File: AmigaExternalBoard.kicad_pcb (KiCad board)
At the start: 2 copper layers, 132.9 x 40.7 mm, 24 parts, among them J1 Conn_01x24, J2 Conn_01x24, J3 Conn_01x24, SW1 SW_SPDT, SW2 SW_SPDT, SW3 SW_SPDT

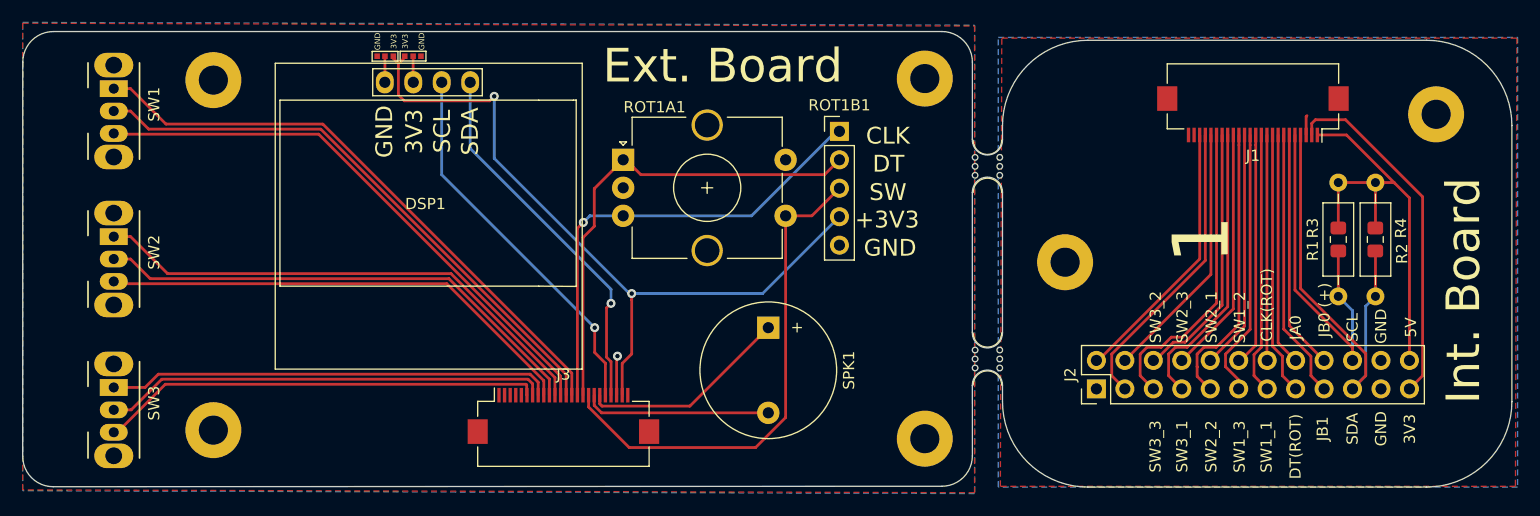
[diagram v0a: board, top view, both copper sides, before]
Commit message: Picture
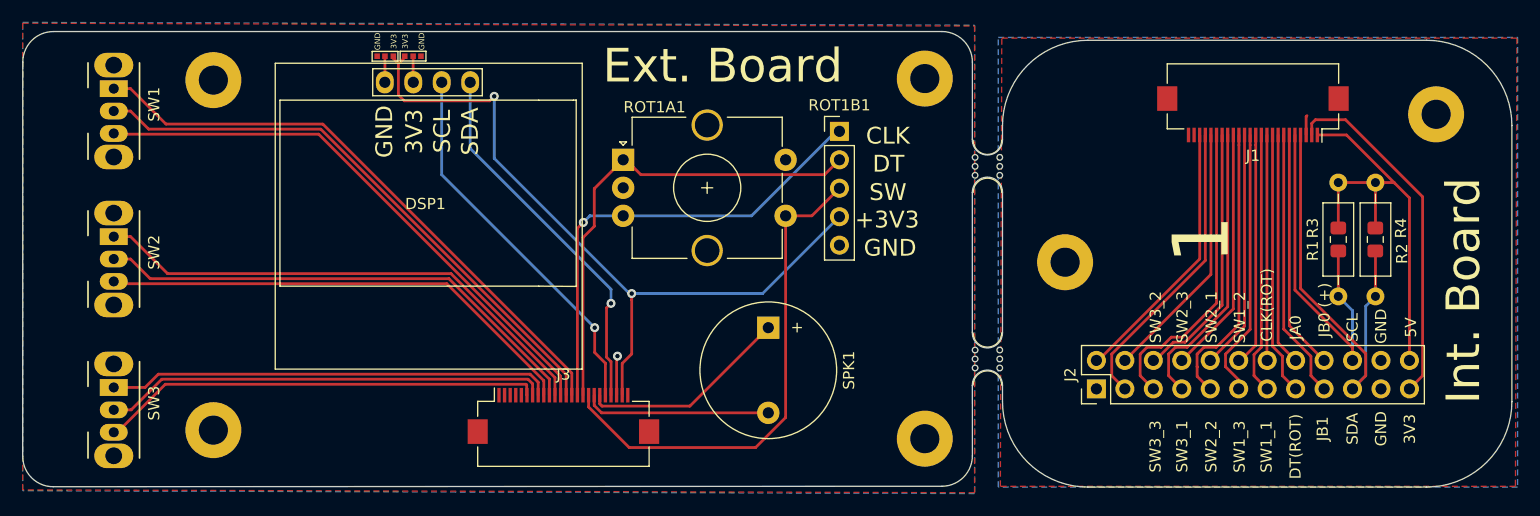
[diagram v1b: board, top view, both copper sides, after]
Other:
- net class 3V3 removed
- net class 5V removed
- net class Default removed
